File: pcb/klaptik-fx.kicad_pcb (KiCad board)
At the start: 4 copper layers, 40.6 x 22.2 mm, 31 parts, among them J1 QWIIC, J2 TagConnect, J4 Conn_01x06, J5 IO_B, J6 IO_A, U1 STM32G0xxFx, U2 LCD12864, U3 M95M01-DF

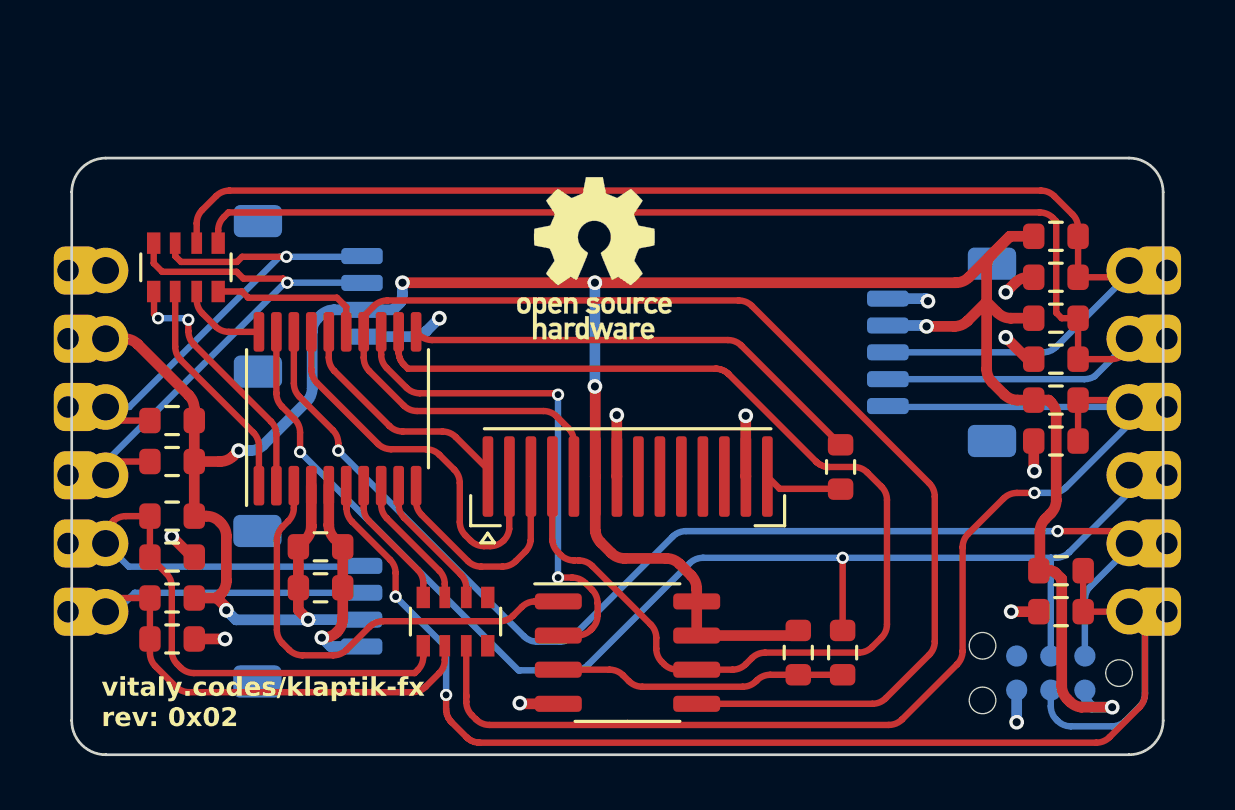
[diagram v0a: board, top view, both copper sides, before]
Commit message: rev 0x03
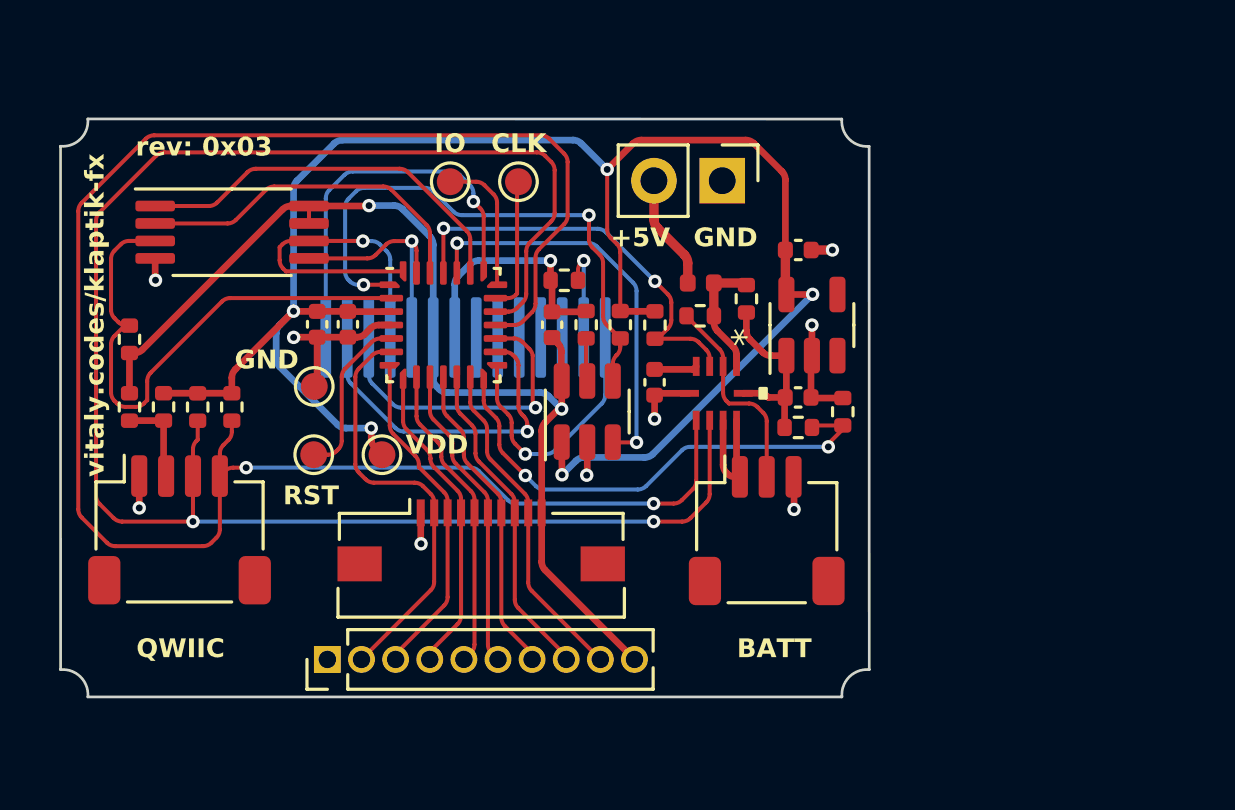
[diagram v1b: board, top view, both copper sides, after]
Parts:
- removed C7, C8: 100nF, Resistor_SMD:R_0603_1608Metric
- removed J6: IO_A, Connector_JST:JST_SH_SM04B-SRSS-TB_1x04-1MP_P1.00mm_Horizontal
- removed RN1, RN2: 190Ω, Resistor_SMD:R_Array_Convex_4x0603
- removed locked: Conn_01x06, Footprints:SolderConnector
- added F1: Polyfuse, Fuse:Fuse_0402_1005Metric, F.Cu at (133.3, 96.5)
- added J3: FFC, Connector_FFC-FPC:Molex_54548-1071_1x10-1MP_P0.5mm_Horizontal, F.Cu at (125.1, 106.1)
- added R12: 0Ω, Resistor_SMD:R_0402_1005Metric, F.Cu at (128.2, 96.4)
- added R13: 10KΩ, Resistor_SMD:R_0402_1005Metric, F.Cu at (112.0, 98.6)
- added TP1: VDD, TestPoint:TestPoint_Pad_D1.0mm, F.Cu at (121.4, 102.9)
- added TP2: GND, TestPoint:TestPoint_Pad_D1.0mm, F.Cu at (118.9, 100.3)
- added TP3: GND, TestPoint:TestPoint_Pad_D1.0mm, F.Cu at (118.9, 102.9)
- added TP4: SWD IO, TestPoint:TestPoint_Pad_D1.0mm, F.Cu at (126.5, 92.7)
- added TP5: SWD CLK, TestPoint:TestPoint_Pad_D1.0mm, F.Cu at (124.0, 92.7)
- added U4: LCD12864, @jb:LCD_FPC_1x14_P0.80mm, B.Cu at (124.5, 98.0)
- added U5: STM32G041G8Ux, Package_DFN_QFN:QFN-28_4x4mm_P0.5mm, F.Cu at (123.7, 98.0)
- added U6: M95512, Package_SO:TSSOP-8_4.4x3mm_P0.65mm, F.Cu at (115.8, 94.6)
- C1: value 10uF -> 4.7uF; footprint Resistor_SMD:R_0603_1608Metric -> Capacitor_SMD:C_0402_1005Metric
- C2, C3, C4, C6: value 100nF -> 4.7uF; footprint Resistor_SMD:R_0603_1608Metric -> Capacitor_SMD:C_0402_1005Metric
- C5: footprint Resistor_SMD:R_0603_1608Metric -> Capacitor_SMD:C_0402_1005Metric
- J1: value QWIIC -> Power; footprint Connector_JST:JST_SH_SM04B-SRSS-TB_1x04-1MP_P1.00mm_Horizontal -> Connector_PinHeader_2.54mm:PinHeader_1x02_P2.54mm_Vertical; moved to F.Cu
- J2: value TagConnect -> BAT; footprint Connector:Tag-Connect_TC2030-IDC-NL_2x03_P1.27mm_Vertical -> Connector_JST:JST_SH_SM03B-SRSS-TB_1x03-1MP_P1.00mm_Horizontal; moved to F.Cu
- J4: value Conn_01x06 -> Header; footprint Footprints:SolderConnector -> Connector_PinHeader_1.27mm:PinHeader_1x10_P1.27mm_Vertical
- J5: value IO_B -> QWIIC; footprint Connector_JST:JST_SH_SM05B-SRSS-TB_1x05-1MP_P1.00mm_Horizontal -> Connector_JST:JST_SH_SM04B-SRSS-TB_1x04-1MP_P1.00mm_Horizontal; moved to F.Cu
- R1: value 4.7KΩ -> 10KΩ; footprint Resistor_SMD:R_0603_1608Metric -> Resistor_SMD:R_0402_1005Metric
- R10: value 10KΩ -> 2.2KΩ; footprint Resistor_SMD:R_0603_1608Metric -> Resistor_SMD:R_0402_1005Metric
- R11: value DNP -> 2.2KΩ; footprint Resistor_SMD:R_0603_1608Metric -> Resistor_SMD:R_0402_1005Metric
- R2: value 4.7KΩ -> DNP; footprint Resistor_SMD:R_0603_1608Metric -> Resistor_SMD:R_0402_1005Metric
- R3: value 10KΩ -> 100KΩ; footprint Resistor_SMD:R_0603_1608Metric -> Resistor_SMD:R_0402_1005Metric
- R4, R6: value 10KΩ -> 20KΩ; footprint Resistor_SMD:R_0603_1608Metric -> Resistor_SMD:R_0402_1005Metric
- R5, R7: footprint Resistor_SMD:R_0603_1608Metric -> Resistor_SMD:R_0402_1005Metric
- R8: value 10KΩ -> 0Ω; footprint Resistor_SMD:R_0603_1608Metric -> Resistor_SMD:R_0402_1005Metric
- R9: value 0Ω -> DNP; footprint Resistor_SMD:R_0603_1608Metric -> Resistor_SMD:R_0402_1005Metric
- REF**: moved to B.Cu
- U1: value STM32G0xxFx -> AP7370-33W5-7; footprint Package_SO:TSSOP-20_4.4x6.5mm_P0.65mm -> Package_TO_SOT_SMD:TSOT-23-5
- U2: value LCD12864 -> AP22652_3x; footprint @jb:LCD_FPC_1x14_P0.80mm -> Package_TO_SOT_SMD:SOT-23-6
- U3: value M95M01-DF -> MP2667GG; footprint Package_SO:SO-8_3.9x4.9mm_P1.27mm -> @jb:MP2667GG-xxxx-Z
- moved R8 35.1 mm to (112.0, 101.1), turned to 90 degrees
- moved J5 29.1 mm to (113.9, 105.7), turned to 0 degrees
- moved R9 25.3 mm to (113.3, 101.1), turned to 90 degrees
- moved R11 24.5 mm to (115.8, 101.1)
- moved R10 24.1 mm to (114.6, 101.1)
- moved R4 23.5 mm to (136.9, 101.9), turned to 0 degrees
- moved R2 22.2 mm to (135.0, 97.1), turned to 90 degrees
- moved R1 20.0 mm to (133.3, 97.7)
- moved R5 19.5 mm to (130.3, 98.0), turned to 90 degrees
- moved C6 19.2 mm to (127.7, 98.0), turned to 90 degrees
- moved C1 19.1 mm to (136.9, 100.7)
- moved U1 17.9 mm to (137.4, 98.0)
- moved R6 17.7 mm to (129.0, 98.0), turned to 90 degrees
- moved R3 17.7 mm to (131.6, 98.0), turned to -90 degrees
- moved REF** 16.7 mm to (113.3, 100.4), turned to 180 degrees
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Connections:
- C1 pad 1: VDD -> VCC
- C2 pad 1: VDD -> Net-(U3-VDD)
- C3 pad 1: /RESET -> VDD
- C4 pad 1: /GPIO_A2 -> VDD
- C5 pad 1: /GPIO_A1 -> VDD
- C6 pad 1: /GPIO_B1 -> Vdrive
- J1 pad 2: VDD -> Net-(J1-Pin_2)
- J2 pad 1: VDD -> /BAT+
- J2 pad 2: /SWD_IO -> Net-(J2-Pin_2)
- J2 pad 3: /RESET -> GND
- J4 pad 2: VDD -> /IO0
- J4 pad 3: /I2C_SCL -> /IO1
- J4 pad 4: /I2C_SDA -> /IO2
- J4 pad 5: /GPIO_A2 -> /IO3
- J4 pad 6: /GPIO_A1 -> /IO4
- J5 pad 2: VDD -> Net-(J5-Pin_2)
- J5 pad 3: /GPIO_B3 -> /I2C_SDA
- J5 pad 4: /GPIO_B2 -> /I2C_SCL
- R1 pad 1: VDD -> /V_{in}
- R1 pad 2: /I2C_SCL -> Net-(J2-Pin_2)
- R10 pad 2: Net-(U3-~{W}) -> /I2C_SDA
- R11 pad 1: /SWD_CLK -> VDD
- R11 pad 2: Net-(U3-~{W}) -> /I2C_SCL
- R2 pad 1: VDD -> VCC
- R2 pad 2: /I2C_SDA -> /V_{in}
- R3 pad 2: /RESET -> /~{PWR_INT}
- R4 pad 1: VDD -> VCC
- R4 pad 2: /GPIO_A2 -> /VCC_SENSE
- R5 pad 1: VDD -> /~{PWR_FLT}
- R5 pad 2: /GPIO_A1 -> VDD
- R6 pad 1: VDD -> Net-(U2-ILIM)
- R6 pad 2: /GPIO_B1 -> GND
- R7 pad 1: VDD -> /VCC_SENSE
- R7 pad 2: /GPIO_B2 -> GND
- R8 pad 1: VDD -> Net-(J5-Pin_2)
- R8 pad 2: /GPIO_B3 -> Vdrive
- R9 pad 1: /LCD_BLK -> Net-(J5-Pin_2)
- R9 pad 2: Net-(U2-LED_A) -> VDD
- U1 pad 1: Net-(RN2-R2.1) -> VCC
- U1 pad 2: Net-(RN2-R1.1) -> GND
- U1 pad 3: /FLASH_CS -> unconnected-(U1-NC-Pad3)
- U1 pad 4: VDD -> unconnected-(U1-NC-Pad4)
- U1 pad 5: GND -> VDD
- U2 pad 1: /LCD_CS -> VDD
- U2 pad 2: /LCD_RESET -> GND
- U2 pad 3: /LCD_A0 -> /PRW_EN
- U2 pad 4: /SPI_CLK -> /~{PWR_FLT}
- U2 pad 5: /SPI_MOSI -> Net-(U2-ILIM)
- U2 pad 6: VDD -> Vdrive
- U3 pad 1: /FLASH_CS -> /V_{in}
- U3 pad 2: /SPI_MISO -> Net-(J2-Pin_2)
- U3 pad 3: Net-(U3-~{W}) -> /~{PWR_INT}
- U3 pad 4: GND -> Net-(U3-VDD)
- U3 pad 5: /SPI_MOSI -> GND
- U3 pad 6: /SPI_CLK -> /I2C_SCL
- U3 pad 7: VDD -> /I2C_SDA
- U3 pad 8: VDD -> /BAT+
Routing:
- net /RESET: track 52.2 -> 0.00 mm, vias 2 -> 0
- net /I2C_SCL: track 18.8 -> 70.1 mm, vias 1 -> 2
- net /GPIO_B2: track 50.1 -> 0.00 mm
- net /GPIO_B3: track 49.0 -> 0.00 mm
- net /GPIO_B1: track 47.4 -> 0.00 mm, vias 1 -> 0
- net /I2C_SDA: track 20.7 -> 65.6 mm, vias 1 -> 2
- net /SWD_CLK: track 48.6 -> 5.18 mm, vias 2 -> 0
- net /SPI_MOSI: track 51.4 -> 8.88 mm, vias 0 -> 1
- net VDD: track 110.2 -> 68.5 mm, vias 8 -> 5
- net Vdrive: track 0.00 -> 40.5 mm, vias 0 -> 2
- net /SWD_IO: track 44.1 -> 5.04 mm, vias 2 -> 0
- net /SPI_CLK: track 44.1 -> 12.8 mm, vias 0 -> 1
- net /GPIO_A2: track 28.2 -> 0.00 mm
- net /GPIO_A1: track 26.5 -> 0.00 mm
- net /~{PWR_FLT}: track 0.00 -> 20.8 mm, vias 0 -> 2
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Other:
- board size 40.6 x 22.2 mm -> 30.1 x 21.5 mm
- board text added: "+5V"
- board text added: "BATT"
- board text added: "CLK"
- board text added: "IO"
- board text added: "VDD"
- board text added: "rev: 0x03"
- board text added: "vitaly.codes/klaptik-fx"
- board text removed: "+3.3V"
- board text removed: "A1"
- board text removed: "A2"
- board text removed: "B1"
- board text removed: "B2"
- board text removed: "B3"
- board text removed: "GPIO A"
- board text removed: "GPIO B"
- board text removed: "I2C CLK"
- board text removed: "I2C SDA"
- board text removed: "SWD"
- board text removed: "SWD CLK"
- board text removed: "SWD IO"
- board text removed: "vitaly.codes/klaptik-fx rev: 0x02"
